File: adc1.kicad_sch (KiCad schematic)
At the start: 42 parts, among them U5 ADS7953QDBTRQ1

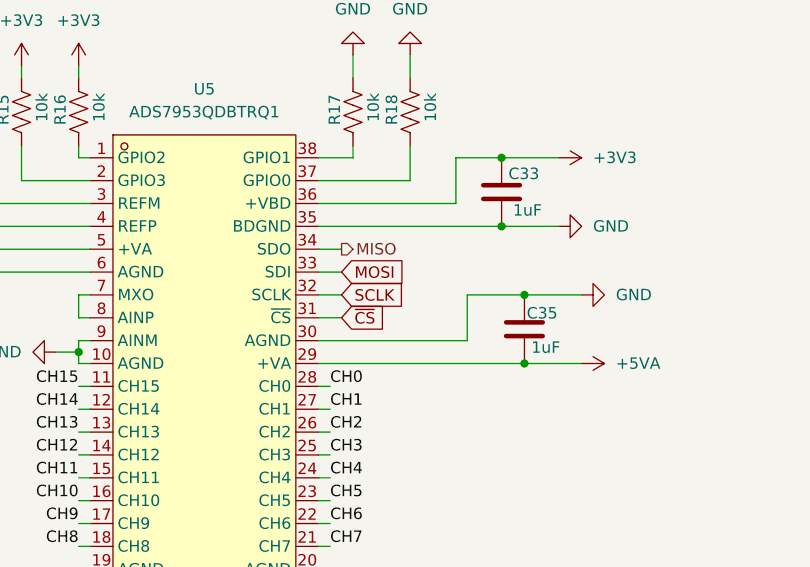
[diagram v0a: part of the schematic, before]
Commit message: PCB layout v1
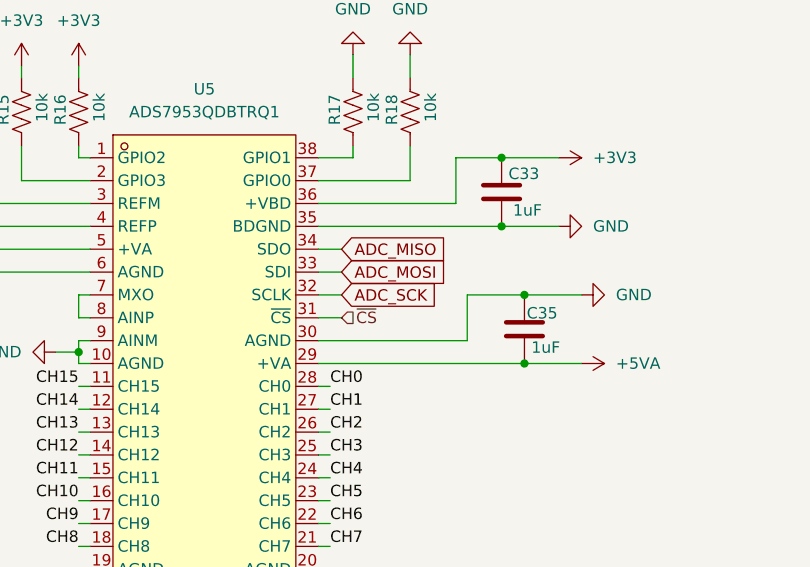
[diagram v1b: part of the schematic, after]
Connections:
- net MISO renamed ADC_MISO
- net MOSI renamed ADC_MOSI
- net SCLK renamed ADC_SCK

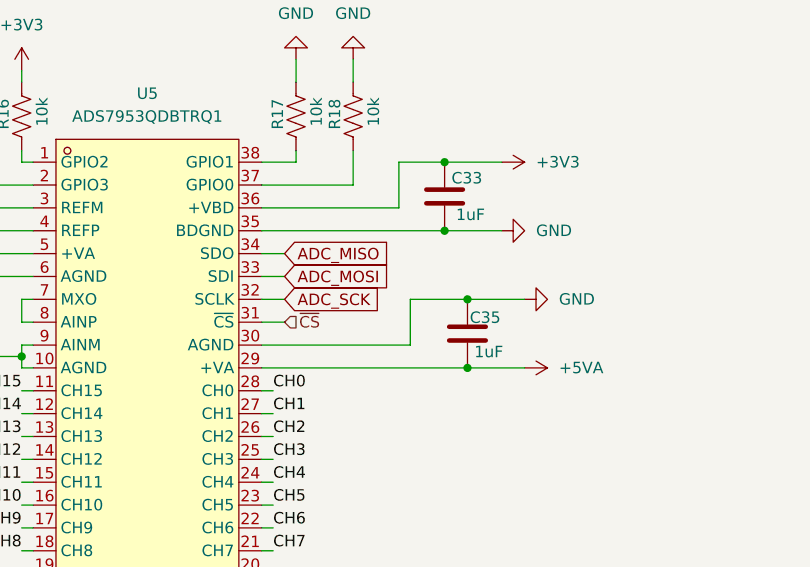
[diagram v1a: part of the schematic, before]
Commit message: progress towards v2
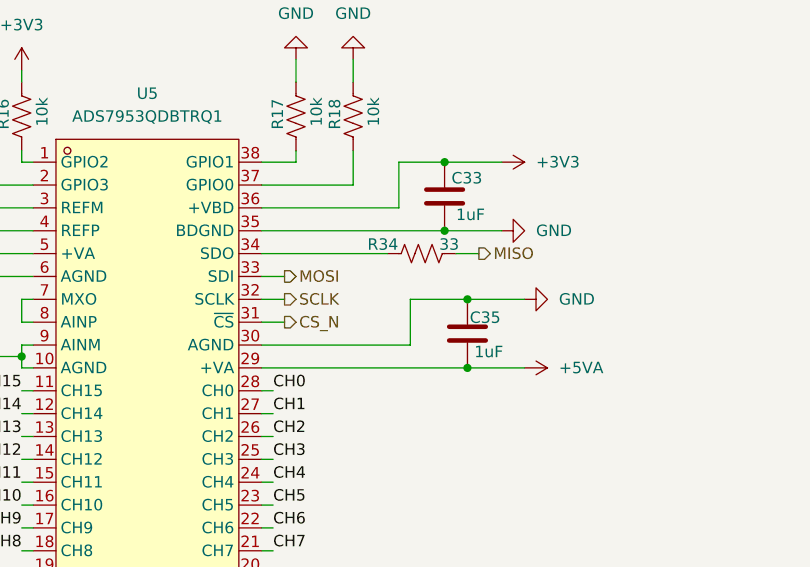
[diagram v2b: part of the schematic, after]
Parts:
- added R34: 33, Resistor_SMD:R_0402_1005Metric, symbol Device:R_US
- R15, R16, R17, R18: footprint Resistor_SMD:R_0603_1608Metric_Pad0.98x0.95mm_HandSolder -> Resistor_SMD:R_0402_1005Metric
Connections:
- net ADC_MISO: no longer names the net of U5.34 (SDO)
- net ADC_MISO: now also R34.1
- net ADC_MOSI renamed MOSI
- net ADC_SCK renamed SCLK
- net ~{CS} renamed CS_N
- new net MISO: R34.2
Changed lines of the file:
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@@
 	(wire
 		(pts
-			(xy 132.08 127) (xy 134.62 127)
+			(xy 132.08 127) (xy 146.05 127)
 		)
 		(stroke
@@
 	(wire
 		(pts
+			(xy 153.67 127) (xy 156.21 127)
+		)
+		(stroke
+			(width 0)
+			(type default)
+		)
+	)
+	(wire
+		(pts
 			(xy 19.05 36.83) (xy 24.13 36.83)
 		)
@@
 		)
 	)
-	(global_label "ADC_MOSI"
+	(global_label "+2V5_REF"
 		(shape input)
-		(at 134.62 129.54 0)
+		(at 76.2 124.46 180)
 		(fields_autoplaced yes)
 		(effects
@@
 				(size 1.27 1.27)
 			)
-			(justify left)
+			(justify right)
 		)
 		(property "Intersheetrefs" "${INTERSHEET_REFS}"
-			(at 146.7976 129.54 0)
+			(at 63.6596 124.46 0)
 			(hide yes)
 			(show_name no)
@@
 					(size 1.27 1.27)
 				)
-				(justify left)
+				(justify right)
 			)
 		)
 	)
-	(global_label "ADC_MISO"
-		(shape input)
-		(at 134.62 127 0)
-		(fields_autoplaced yes)
+	(hierarchical_label "MISO"
+		(shape output)
+		(at 156.21 127 0)
 		(effects
 			(font
@@
 			(justify left)
 		)
-		(property "Intersheetrefs" "${INTERSHEET_REFS}"
-			(at 146.7976 127 0)
-			(hide yes)
-			(show_name no)
-			(do_not_autoplace no)
-			(effects
-				(font
-					(size 1.27 1.27)
-				)
-				(justify left)
-			)
-		)
 	)
-	(global_label "ADC_SCK"
-		(shape input)
-		(at 134.62 132.08 0)
-		(fields_autoplaced yes)
+	(hierarchical_label "CS_N"
+		(shape output)
+		(at 134.62 134.62 0)
 		(effects
 			(font
@@
 			(justify left)
 		)
-		(property "Intersheetrefs" "${INTERSHEET_REFS}"
-			(at 145.9509 132.08 0)
-			(hide yes)
-			(show_name no)
-			(do_not_autoplace no)
-			(effects
-				(font
-					(size 1.27 1.27)
-				)
-				(justify left)
-			)
-		)
 	)
-	(global_label "+2V5_REF"
-		(shape input)
-		(at 76.2 124.46 180)
-		(fields_autoplaced yes)
+	(hierarchical_label "MOSI"
+		(shape output)
+		(at 134.62 129.54 0)
 		(effects
 			(font
 				(size 1.27 1.27)
 			)
-			(justify right)
-		)
-		(property "Intersheetrefs" "${INTERSHEET_REFS}"
-			(at 63.6596 124.46 0)
-			(hide yes)
-			(show_name no)
-			(do_not_autoplace no)
-			(effects
-				(font
-					(size 1.27 1.27)
-				)
-				(justify right)
-			)
+			(justify left)
 		)
 	)
-	(hierarchical_label "~{CS}"
-		(shape input)
-		(at 134.62 134.62 0)
+	(hierarchical_label "SCLK"
+		(shape output)
+		(at 134.62 132.08 0)
 		(effects
 			(font
@@
 			)
 		)
-		(property "Footprint" "Resistor_SMD:R_0603_1608Metric_Pad0.98x0.95mm_HandSolder"
+		(property "Footprint" "Resistor_SMD:R_0402_1005Metric"
 			(at 134.874 111.506 90)
 			(hide yes)
@@
 	(symbol
 		(lib_id "Device:R_US")
+		(at 149.86 127 90)
+		(unit 1)
+		(body_style 1)
+		(exclude_from_sim no)
+		(in_bom yes)
+		(on_board yes)
+		(in_pos_files yes)
+		(dnp no)
+		(property "Reference" "R34"
+			(at 145.542 125.984 90)
+			(show_name no)
+			(do_not_autoplace no)
+			(effects
+				(font
+					(size 1.27 1.27)
+				)
+			)
+		)
+		(property "Value" "33"
+			(at 152.908 125.984 90)
+			(show_name no)
+			(do_not_autoplace no)
+			(effects
+				(font
+					(size 1.27 1.27)
+				)
+			)
+		)
+		(property "Footprint" "Resistor_SMD:R_0402_1005Metric"
+			(at 150.114 125.984 90)
+			(hide yes)
+			(show_name no)
+			(do_not_autoplace no)
+			(effects
+				(font
+					(size 1.27 1.27)
+				)
+			)
+		)
+		(property "Datasheet" ""
+			(at 149.86 127 0)
+			(hide yes)
+			(show_name no)
+			(do_not_autoplace no)
+			(effects
+				(font
+					(size 1.27 1.27)
+				)
+			)
+		)
+		(property "Description" "Resistor, US symbol"
+			(at 149.86 127 0)
+			(hide yes)
+			(show_name no)
+			(do_not_autoplace no)
+			(effects
+				(font
+					(size 1.27 1.27)
+				)
+			)
+		)
+		(property "LCSC Part" "C23140"
+			(at 149.86 127 90)
+			(hide yes)
+			(show_name no)
+			(do_not_autoplace no)
+			(effects
+				(font
+					(size 1.27 1.27)
+				)
+			)
+		)
+		(pin "2"
+		)
+		(pin "1"
+		)
+		(instances
+			(project "stav-keeb-65"
+				(path "/f067c205-942c-45af-b694-038ca43c147c/102b9583-fe1e-454e-b472-c731d3a32681"
+					(reference "R37")
+					(unit 1)
+				)
+				(path "/f067c205-942c-45af-b694-038ca43c147c/7ed9120e-f11c-4b22-935f-1ee89d31afd6"
+					(reference "R34")
+					(unit 1)
+				)
+				(path "/f067c205-942c-45af-b694-038ca43c147c/a1b97858-44bd-4201-b050-5e153f225d6a"
+					(reference "R36")
+					(unit 1)
+				)
+				(path "/f067c205-942c-45af-b694-038ca43c147c/c1663012-812f-4121-9717-99888f6b08f2"
+					(reference "R35")
+					(unit 1)
+				)
+			)
+		)
+	)
+	(symbol
+		(lib_id "Device:R_US")
 		(at 105.41 111.76 180)
 		(unit 1)
@@
 			)
 		)
-		(property "Footprint" "Resistor_SMD:R_0603_1608Metric_Pad0.98x0.95mm_HandSolder"
+		(property "Footprint" "Resistor_SMD:R_0402_1005Metric"
 			(at 104.394 111.506 90)
 			(hide yes)
@@
 			)
 		)
-		(property "Footprint" "Resistor_SMD:R_0603_1608Metric_Pad0.98x0.95mm_HandSolder"
+		(property "Footprint" "Resistor_SMD:R_0402_1005Metric"
 			(at 141.224 111.506 90)
 			(hide yes)
@@
 			)
 		)
-		(property "Footprint" "Resistor_SMD:R_0603_1608Metric_Pad0.98x0.95mm_HandSolder"
+		(property "Footprint" "Resistor_SMD:R_0402_1005Metric"
 			(at 98.044 111.506 90)
 			(hide yes)

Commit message: more progress towards v2
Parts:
- C31, C32, C33, C34, C35, K_C1, K_C10, K_C11, K_C12, K_C13, K_C14, K_C15, K_C16, K_C2, K_C3, K_C4, K_C5, K_C6, K_C7, K_C8, K_C9: footprint Capacitor_SMD:C_0603_1608Metric_Pad1.08x0.95mm_HandSolder -> Capacitor_SMD:C_0402_1005Metric
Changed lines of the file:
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@@
 			)
 		)
-		(property "Footprint" "Capacitor_SMD:C_0603_1608Metric_Pad1.08x0.95mm_HandSolder"
+		(property "Footprint" "Capacitor_SMD:C_0402_1005Metric"
 			(at 80.9752 124.46 0)
 			(hide yes)
@@
 			)
 		)
-		(property "Footprint" "Capacitor_SMD:C_0603_1608Metric_Pad1.08x0.95mm_HandSolder"
+		(property "Footprint" "Capacitor_SMD:C_0402_1005Metric"
 			(at 75.2348 73.66 0)
 			(hide yes)
@@
 			)
 		)
-		(property "Footprint" "Capacitor_SMD:C_0603_1608Metric_Pad1.08x0.95mm_HandSolder"
+		(property "Footprint" "Capacitor_SMD:C_0402_1005Metric"
 			(at 49.8348 38.1 0)
 			(hide yes)
@@
 			)
 		)
-		(property "Footprint" "Capacitor_SMD:C_0603_1608Metric_Pad1.08x0.95mm_HandSolder"
+		(property "Footprint" "Capacitor_SMD:C_0402_1005Metric"
 			(at 207.3148 38.1 0)
 			(hide yes)
@@
 			)
 		)
-		(property "Footprint" "Capacitor_SMD:C_0603_1608Metric_Pad1.08x0.95mm_HandSolder"
+		(property "Footprint" "Capacitor_SMD:C_0402_1005Metric"
 			(at 86.6648 116.84 0)
 			(hide yes)
@@
 			)
 		)
-		(property "Footprint" "Capacitor_SMD:C_0603_1608Metric_Pad1.08x0.95mm_HandSolder"
+		(property "Footprint" "Capacitor_SMD:C_0402_1005Metric"
 			(at 155.9052 139.7 0)
 			(hide yes)
@@
 			)
 		)
-		(property "Footprint" "Capacitor_SMD:C_0603_1608Metric_Pad1.08x0.95mm_HandSolder"
+		(property "Footprint" "Capacitor_SMD:C_0402_1005Metric"
 			(at 75.2348 38.1 0)
 			(hide yes)
@@
 			)
 		)
-		(property "Footprint" "Capacitor_SMD:C_0603_1608Metric_Pad1.08x0.95mm_HandSolder"
+		(property "Footprint" "Capacitor_SMD:C_0402_1005Metric"
 			(at 101.9048 73.66 0)
 			(hide yes)
@@
 			)
 		)
-		(property "Footprint" "Capacitor_SMD:C_0603_1608Metric_Pad1.08x0.95mm_HandSolder"
+		(property "Footprint" "Capacitor_SMD:C_0402_1005Metric"
 			(at 23.1648 73.66 0)
 			(hide yes)
@@
 			)
 		)
-		(property "Footprint" "Capacitor_SMD:C_0603_1608Metric_Pad1.08x0.95mm_HandSolder"
+		(property "Footprint" "Capacitor_SMD:C_0402_1005Metric"
 			(at 155.2448 73.66 0)
 			(hide yes)
@@
 			)
 		)
-		(property "Footprint" "Capacitor_SMD:C_0603_1608Metric_Pad1.08x0.95mm_HandSolder"
+		(property "Footprint" "Capacitor_SMD:C_0402_1005Metric"
 			(at 88.5952 134.62 0)
 			(hide yes)
@@
 			)
 		)
-		(property "Footprint" "Capacitor_SMD:C_0603_1608Metric_Pad1.08x0.95mm_HandSolder"
+		(property "Footprint" "Capacitor_SMD:C_0402_1005Metric"
 			(at 153.3652 124.46 0)
 			(hide yes)
@@
 			)
 		)
-		(property "Footprint" "Capacitor_SMD:C_0603_1608Metric_Pad1.08x0.95mm_HandSolder"
+		(property "Footprint" "Capacitor_SMD:C_0402_1005Metric"
 			(at 49.8348 73.66 0)
 			(hide yes)
@@
 			)
 		)
-		(property "Footprint" "Capacitor_SMD:C_0603_1608Metric_Pad1.08x0.95mm_HandSolder"
+		(property "Footprint" "Capacitor_SMD:C_0402_1005Metric"
 			(at 155.2448 38.1 0)
 			(hide yes)
@@
 			)
 		)
-		(property "Footprint" "Capacitor_SMD:C_0603_1608Metric_Pad1.08x0.95mm_HandSolder"
+		(property "Footprint" "Capacitor_SMD:C_0402_1005Metric"
 			(at 128.5748 73.66 0)
 			(hide yes)
@@
 			)
 		)
-		(property "Footprint" "Capacitor_SMD:C_0603_1608Metric_Pad1.08x0.95mm_HandSolder"
+		(property "Footprint" "Capacitor_SMD:C_0402_1005Metric"
 			(at 180.6448 73.66 0)
 			(hide yes)
@@
 			)
 		)
-		(property "Footprint" "Capacitor_SMD:C_0603_1608Metric_Pad1.08x0.95mm_HandSolder"
+		(property "Footprint" "Capacitor_SMD:C_0402_1005Metric"
 			(at 23.1648 38.1 0)
 			(hide yes)
@@
 			)
 		)
-		(property "Footprint" "Capacitor_SMD:C_0603_1608Metric_Pad1.08x0.95mm_HandSolder"
+		(property "Footprint" "Capacitor_SMD:C_0402_1005Metric"
 			(at 128.5748 38.1 0)
 			(hide yes)
@@
 			)
 		)
-		(property "Footprint" "Capacitor_SMD:C_0603_1608Metric_Pad1.08x0.95mm_HandSolder"
+		(property "Footprint" "Capacitor_SMD:C_0402_1005Metric"
 			(at 180.6448 38.1 0)
 			(hide yes)
@@
 			)
 		)
-		(property "Footprint" "Capacitor_SMD:C_0603_1608Metric_Pad1.08x0.95mm_HandSolder"
+		(property "Footprint" "Capacitor_SMD:C_0402_1005Metric"
 			(at 207.3148 73.66 0)
 			(hide yes)
@@
 			)
 		)
-		(property "Footprint" "Capacitor_SMD:C_0603_1608Metric_Pad1.08x0.95mm_HandSolder"
+		(property "Footprint" "Capacitor_SMD:C_0402_1005Metric"
 			(at 101.9048 38.1 0)
 			(hide yes)
